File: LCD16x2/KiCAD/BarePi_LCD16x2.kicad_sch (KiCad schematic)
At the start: 17 parts, among them J1 IN, J2 OUT, J3 Backlight, J4 WCH-LINK, SW1 VO_DN, SW2 VO_UP, U1 CH32V002A4M6, U2 DM1602A

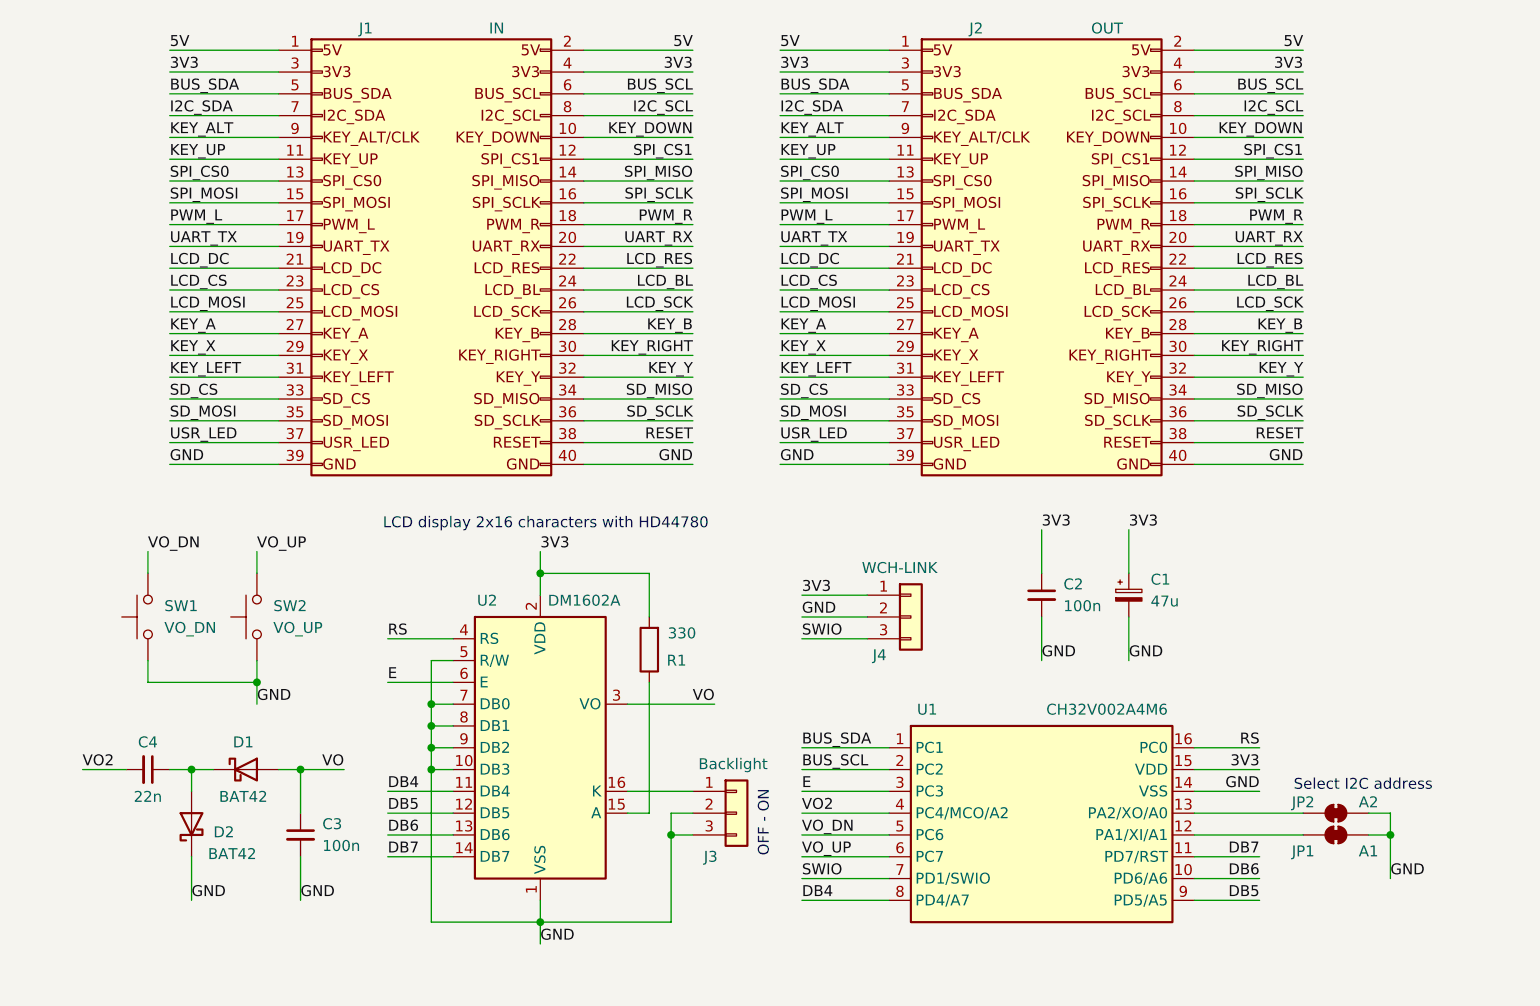
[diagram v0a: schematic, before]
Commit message: init
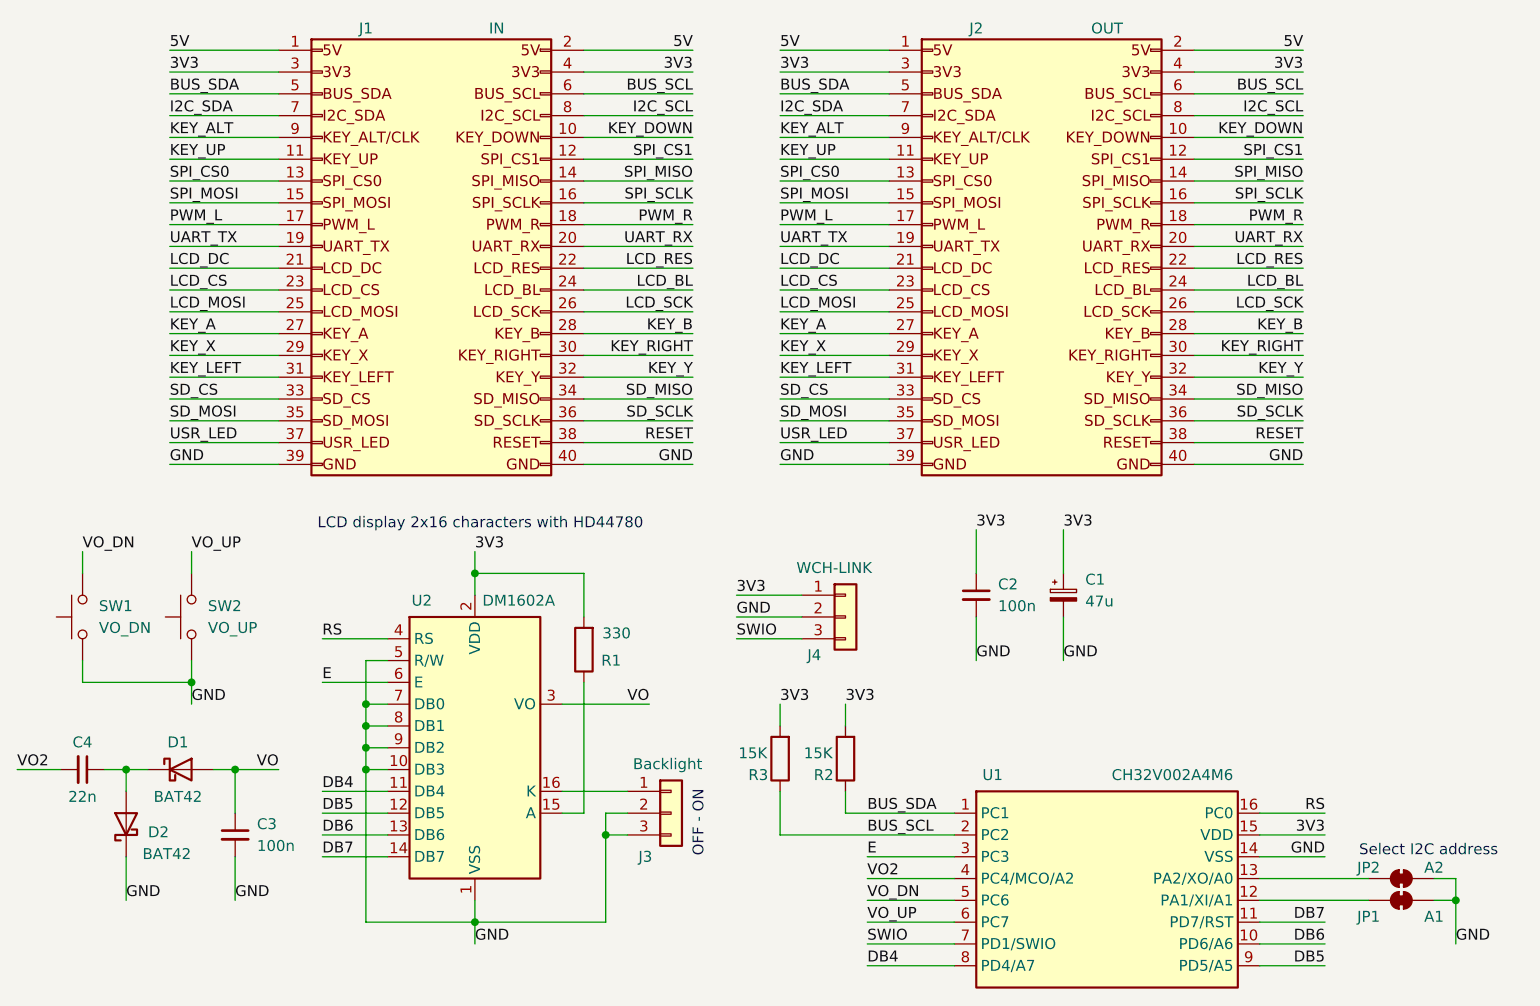
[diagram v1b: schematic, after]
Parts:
- added R2, R3: 15K, Resistor_SMD:R_1206_3216Metric_Pad1.30x1.75mm_HandSolder, symbol Device:R
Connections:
- net 3V3: now also R2.2, R3.2
- net BUS_SCL: now also R3.1
- net BUS_SDA: now also R2.1
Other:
- moved on the sheet: C1, C2, C3, C4, D1, D2, J3, J4, JP1, JP2, R1, SW1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
